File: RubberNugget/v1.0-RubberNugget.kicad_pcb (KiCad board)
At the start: 2 copper layers, 36 x 50 mm, 54 parts, among them J1 Micro USB, J2 JST PH 2.0, J3 JST_SH_SM03B-SRSS-TB_1x03-1MP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, Q1 UMH3N, Q2 DMG3415, SW1 SPDT, SW2 UP, SW3 Reset, SW4 DOWN, SW5 LEFT, SW6 RIGHT, U1 CP2102N-A01-GQFN24, U2 SH1106, U3 MCP73831-2-OT, U4 ESP-12F, U5 AP2112K-3.3

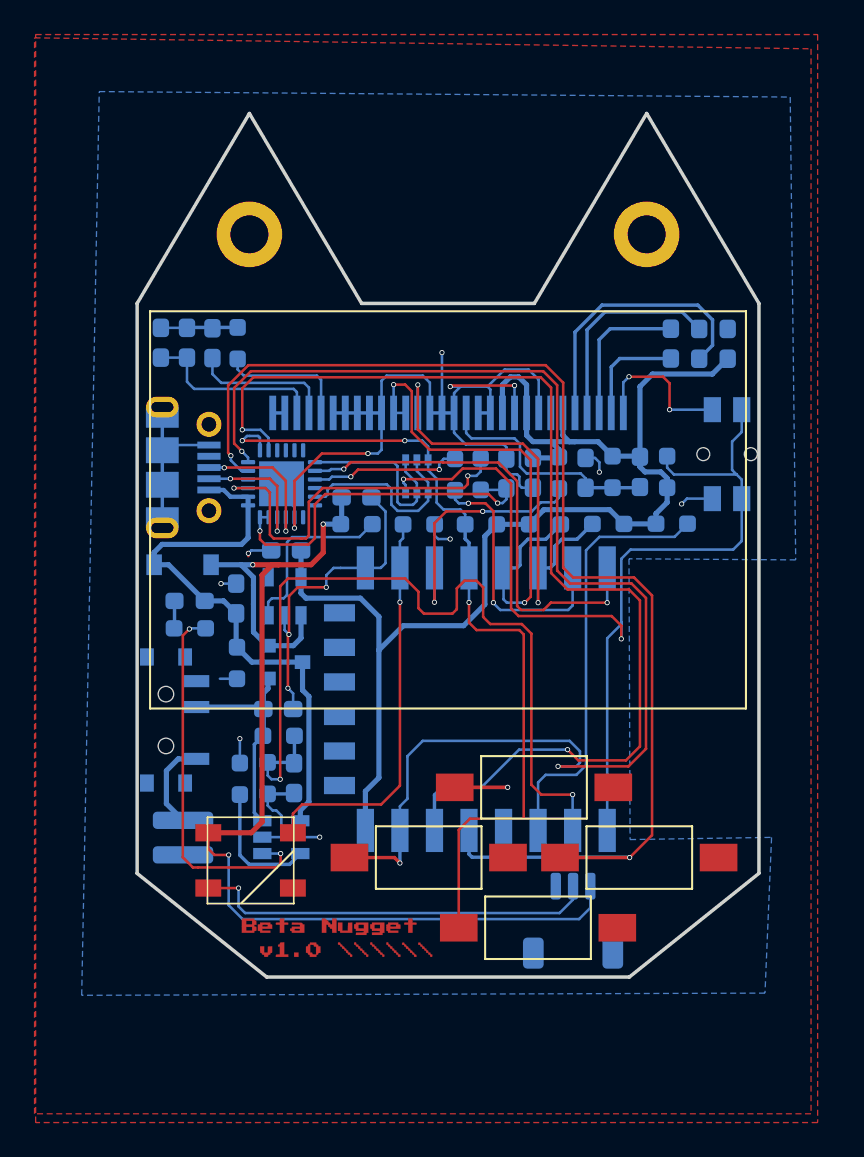
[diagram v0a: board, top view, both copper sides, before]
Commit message: update and re-wire v1.0 alpha
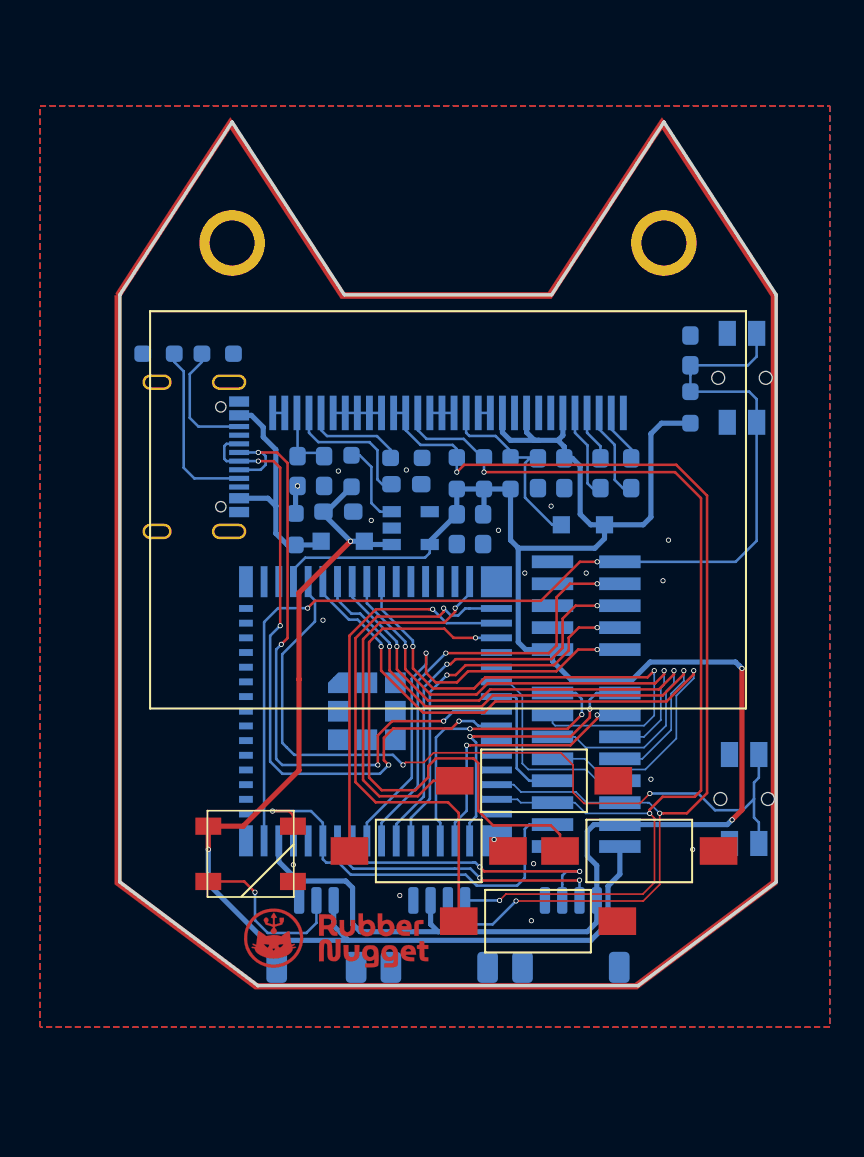
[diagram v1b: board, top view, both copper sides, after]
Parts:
- removed the C10 at (-9.83, 6.99)
- removed C13: 4.7μF, Capacitor_SMD:C_0603_1608Metric_Pad1.08x0.95mm_HandSolder
- removed the C8 at (-12.3, 0.58)
- removed the C9 at (-8.92, 11.0)
- removed the D1 at (11.1, -6.74)
- removed Q1: UMH3N, Package_TO_SOT_SMD:SOT-363_SC-70-6
- removed Q2: DMG3415, Package_TO_SOT_SMD:SOT-23
- removed R10, R14, R15: 10K, Resistor_SMD:R_0603_1608Metric_Pad0.98x0.95mm_HandSolder
- removed R13: 4.7K, Resistor_SMD:R_0603_1608Metric_Pad0.98x0.95mm_HandSolder
- removed R16: 1K, Resistor_SMD:R_0603_1608Metric_Pad0.98x0.95mm_HandSolder
- removed R17: R_Small_US, Resistor_SMD:R_0603_1608Metric_Pad0.98x0.95mm_HandSolder
- removed the R5 at (-9.80, 8.53)
- removed the R6 at (-12.1, 11.0)
- removed the R7 at (-10.4, 11.0)
- removed the R8 at (-14.9, 2.31)
- removed the R9 at (12.7, -6.75)
- removed the REF** at (-11.5, -20.5)
- removed the REF** at (11.5, -20.5)
- removed the Ref** at (0.00, 0.00)
- removed the SW3 at (16.2, -7.77)
- removed the U3 at (-9.65, 14.4)
- removed U4: ESP-12F, RF_Module:ESP-12E
- added ?: , , F.Cu at (25.8, -0.00)
- added C1: 1uF, Capacitor_SMD:C_0603_1608Metric_Pad1.08x0.95mm_HandSolder, B.Cu at (14.0, -13.8)
- added J4: Nugget Expansion, Connector_PinHeader_1.27mm:PinHeader_2x08_P1.27mm_Vertical_SMD, B.Cu at (8.00, 10.5)
- added J5: UART, Connector_JST:JST_SH_SM04B-SRSS-TB_1x04-1MP_P1.00mm_Horizontal, B.Cu at (7.11, 20.1)
- added J6: JTAG, Connector_PinHeader_1.27mm:PinHeader_2x05_P1.27mm_Vertical_SMD, B.Cu at (8.00, 1.00)
- added R1: 5.1K, Resistor_SMD:R_0603_1608Metric_Pad0.98x0.95mm_HandSolder, B.Cu at (-16.8, -13.6)
- added R2: 5.1K, Resistor_SMD:R_0603_1608Metric_Pad0.98x0.95mm_HandSolder, B.Cu at (-13.3, -13.6)
- added R3: 10K, Resistor_SMD:R_0603_1608Metric_Pad0.98x0.95mm_HandSolder, B.Cu at (14.0, -10.5)
- added REF**: MountingHole_2.2mm_M2_DIN965_Pad, MountingHole:MountingHole_2.2mm_M2_DIN965_Pad, F.Cu at (-12.3, -20.1)
- added Ref**: Val**, art, F.Cu at (0.00, 0.20)
- added SW2: Reset, Button_Switch_SMD:Panasonic_EVQPUM_EVQPUD, B.Cu at (17.0, -12.2)
- C10: renamed from C6; value 1 μF -> 1uF
- C3: value 1 μF -> 4.7μF
- C7: value C_Small -> 1uF
- C8: renamed from C14; value C_Small -> 1uF
- C9: renamed from C5; value 1 μF -> 1uF
- D2: value RED -> SS14; footprint LED_SMD:LED_0603_1608Metric_Pad1.05x0.95mm_HandSolder -> Diode_SMD:D_SOD-323_HandSoldering
- D3: footprint Diode_SMD:D_SOD-123 -> Diode_SMD:D_SOD-323_HandSoldering
- J1: value Micro USB -> USB C 2.0; footprint Connector_USB:USB_Micro-B_Molex-105017-0001 -> Connector_USB:USB_C_Receptacle_Palconn_UTC16-G
- J2: value JST PH 2.0 -> QWIIC; footprint Connector_JST:JST_PH_S2B-PH-SM4-TB_1x02-1MP_P2.00mm_Horizontal -> Connector_JST:JST_SH_SM04B-SRSS-TB_1x04-1MP_P1.00mm_Horizontal
- J3: value JST_SH_SM03B-SRSS-TB_1x03-1MP_P1.00mm_Horizontal -> NeoPixel Breakout
- SW1: value SPDT -> Reset; footprint Button_Switch_SMD:SW_SPDT_PCM12 -> Button_Switch_SMD:Panasonic_EVQPUM_EVQPUD
- U1: value CP2102N-A01-GQFN24 -> ESP32-S2-MINI-2; footprint Package_DFN_QFN:QFN-24-1EP_4x4mm_P0.5mm_EP2.6x2.6mm -> Espressif:ESP32-S2-MINI-1_Hand-Soldering
- U3: renamed from U5; value AP2112K-3.3 -> AP2112K / RT9080
- moved SW1 33.5 mm to (17.1, 12.2)
- moved D3 23.3 mm to (7.81, -3.68)
- moved J3 14.9 mm to (-7.62, 20.1)
- moved U1 14.1 mm to (-4.70, 7.11), turned to 270 degrees
- moved C11 13.9 mm to (-2.41, -6.03), turned to 0 degrees
- moved J2 13.2 mm to (-0.51, 20.1), turned to 180 degrees
- moved C6 12.1 mm to (6.73, -6.67), turned to 270 degrees
- moved R9 11.8 mm to (-2.41, -7.56), turned to 0 degrees
- moved C2 11.5 mm to (2.03, -3.43), turned to 270 degrees
- moved C7 10.9 mm to (-7.18, -6.79), turned to 90 degrees
- moved C8 10.9 mm to (-8.71, -6.79), turned to 90 degrees
- moved D2 9.51 mm to (-6.10, -2.73), turned to 180 degrees
- moved C10 9.42 mm to (8.83, -6.67)
- moved R5 8.46 mm to (-8.83, -3.43), turned to 90 degrees
- moved U3 8.30 mm to (-2.16, -3.49), turned to 0 degrees
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- renumbered C4 to C11, C12 to C2, C11 to C4, C2 to C5, C1 to C6, D4 to D1, R12 to R4, R11 to R5, R1 to R6, R2 to R7, R3 to R8, R4 to R9, SW2 to SW3
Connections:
- C11 pad 2: GNDREF -> GND
- C2 pad 2: GNDREF -> GND
- C3 pad 1: GNDREF -> +3V3
- C3 pad 2: Net-(C3-Pad2) -> GND
- C4 pad 2: GNDREF -> GND
- C5 pad 2: GNDREF -> GND
- C6 pad 2: GNDREF -> GND
- C7 pad 1: GNDREF -> GND
- C8 pad 1: GNDREF -> GND
- D1 pad 3: GNDREF -> GND
- D1 pad 4: GPIO15 -> NEOPIXEL
- D2 pad 1: Net-(D2-Pad1) -> VMAX
- D3 pad 1: VMAX -> +3V3
- D3 pad 2: VBUS -> RES
- J2 pad 1: Net-(J2-Pad1) -> SCL
- J2 pad 2: GNDREF -> SDA
- J3 pad 3: GNDREF -> GND
- R5 pad 2: GNDREF -> GND
- R9 pad 2: GNDREF -> GND
- SW1 pad 1: Net-(J2-Pad1) -> BOOT
- SW1 pad 2: +BATT -> GND
- SW3 pad 1: GPIO12 -> UP_BTN
- SW3 pad 2: GNDREF -> GND
- SW4 pad 1: GPIO0 -> DN_BTN
- SW4 pad 2: GNDREF -> GND
- SW5 pad 1: GPIO13 -> LT_BTN
- SW5 pad 2: GNDREF -> GND
- SW6 pad 1: GPIO14 -> RT_BTN
- SW6 pad 2: GNDREF -> GND
- U1 pad 1: Net-(U1-Pad1) -> GND
- U1 pad 11: GPIO14 -> Net-(U1-Pad11)
- U1 pad 12: GPIO13 -> Net-(U1-Pad12)
- U1 pad 13: GPIO0 -> Net-(U1-Pad13)
- U1 pad 14: GPIO12 -> Net-(U1-Pad14)
- U1 pad 15: Net-(U1-Pad15) -> UP_BTN
- U1 pad 16: Net-(U1-Pad16) -> DN_BTN
- U1 pad 17: Net-(U1-Pad17) -> LT_BTN
- U1 pad 18: Net-(U1-Pad18) -> RT_BTN
- U1 pad 19: RTS -> Net-(U1-Pad19)
- U1 pad 2: GNDREF -> GND
- U1 pad 20: TXD -> Net-(U1-Pad20)
- U1 pad 21: USB_RX -> A1
- U1 pad 22: Net-(U1-Pad22) -> A0
- U1 pad 23: DTR -> USB_D-
- U1 pad 24: Net-(U1-Pad24) -> USB_D+
- U1 pad 25: GNDREF -> Net-(U1-Pad25)
- U1 pad 3: Net-(J1-Pad3) -> +3V3
- U1 pad 4: Net-(J1-Pad2) -> BOOT
- U1 pad 5: Net-(C3-Pad2) -> A2
- U1 pad 6: Net-(C3-Pad2) -> A3
- U1 pad 7: VBUS -> A4
- U1 pad 8: VBUS -> A5
- U1 pad 9: Net-(R17-Pad1) -> A6
- U2 pad 1: GNDREF -> GND
- U2 pad 10: GNDREF -> GND
- U2 pad 12: GNDREF -> GND
- U2 pad 13: GNDREF -> GND
- U2 pad 15: GNDREF -> GND
- U2 pad 16: GNDREF -> GND
- U2 pad 17: GNDREF -> GND
- U2 pad 21: GNDREF -> GND
- U2 pad 22: GNDREF -> GND
- U2 pad 23: GNDREF -> GND
- U2 pad 24: GNDREF -> GND
- U2 pad 25: GNDREF -> GND
- U2 pad 29: GNDREF -> GND
- U2 pad 30: GNDREF -> GND
- U2 pad 8: GNDREF -> GND
- U3 pad 2: GNDREF -> GND
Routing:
- net GNDREF: track 113.2 -> 0.00 mm, vias 17 -> 0
- net GPIO13: track 76.9 -> 0.00 mm, vias 3 -> 0
- net GPIO14: track 73.0 -> 0.00 mm, vias 2 -> 0
- net GPIO12: track 68.4 -> 0.00 mm, vias 3 -> 0
- net RST: track 0.00 -> 62.3 mm, vias 0 -> 2
- net ESP_RST: track 59.8 -> 0.00 mm, vias 2 -> 0
- net GPIO0: track 48.4 -> 0.00 mm, vias 3 -> 0
- net BOOT: track 0.00 -> 46.9 mm, vias 0 -> 2
- net +3V3: track 75.6 -> 121.0 mm, vias 0 -> 2
- net A0: track 49.2 -> 7.62 mm, vias 2 -> 0
- net SDA: track 29.9 -> 70.9 mm, vias 2 -> 3
- net A2: track 0.00 -> 39.6 mm, vias 0 -> 2
- net USB_D+: track 0.00 -> 38.4 mm, vias 0 -> 4
- net USB_D-: track 0.00 -> 38.4 mm, vias 0 -> 4
- net SCL: track 27.0 -> 64.9 mm, vias 2 -> 3
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- added copper zone on B.Cu, net (none)
- added copper zone on B.Cu, net GND
- added copper zone on F.Cu, net GND
- removed copper zone on B.Cu, net GNDREF
- removed copper zone on F.Cu, net GNDREF
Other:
- board size 36 x 50 mm -> 38 x 50 mm
- board text added: "v1.0-alpha"
- board text removed: "+"
- board text removed: "-"
